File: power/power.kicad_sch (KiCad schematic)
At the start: 2 parts, among them J1 ET60T-D04-3-08-D04-X-R1-S, J2 796636-6

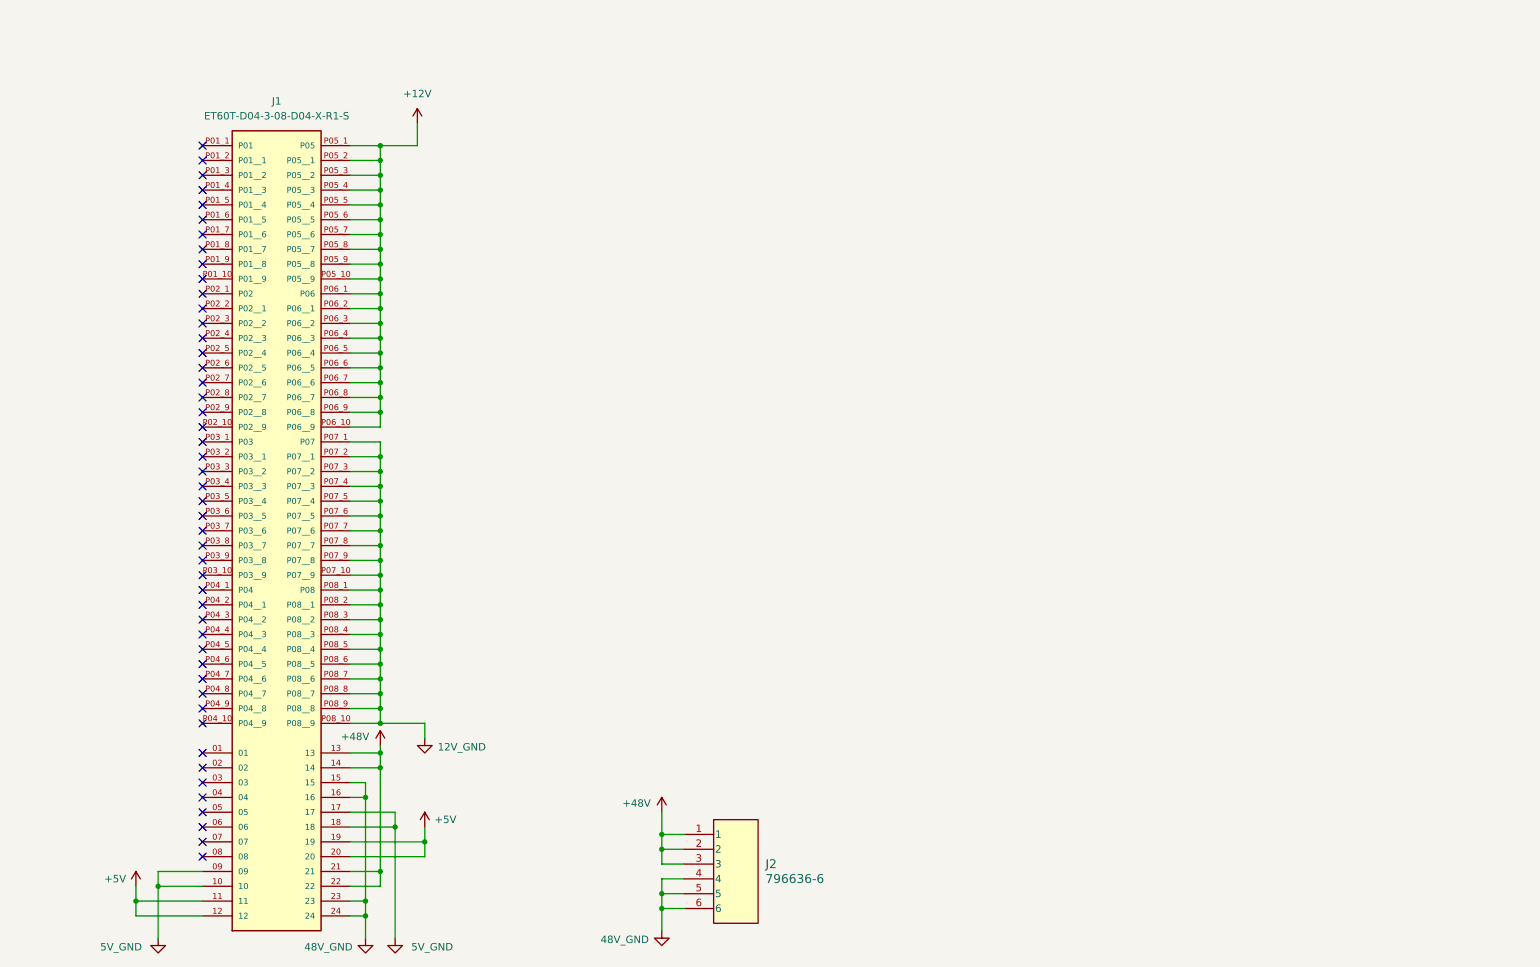
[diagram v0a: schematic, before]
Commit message: work
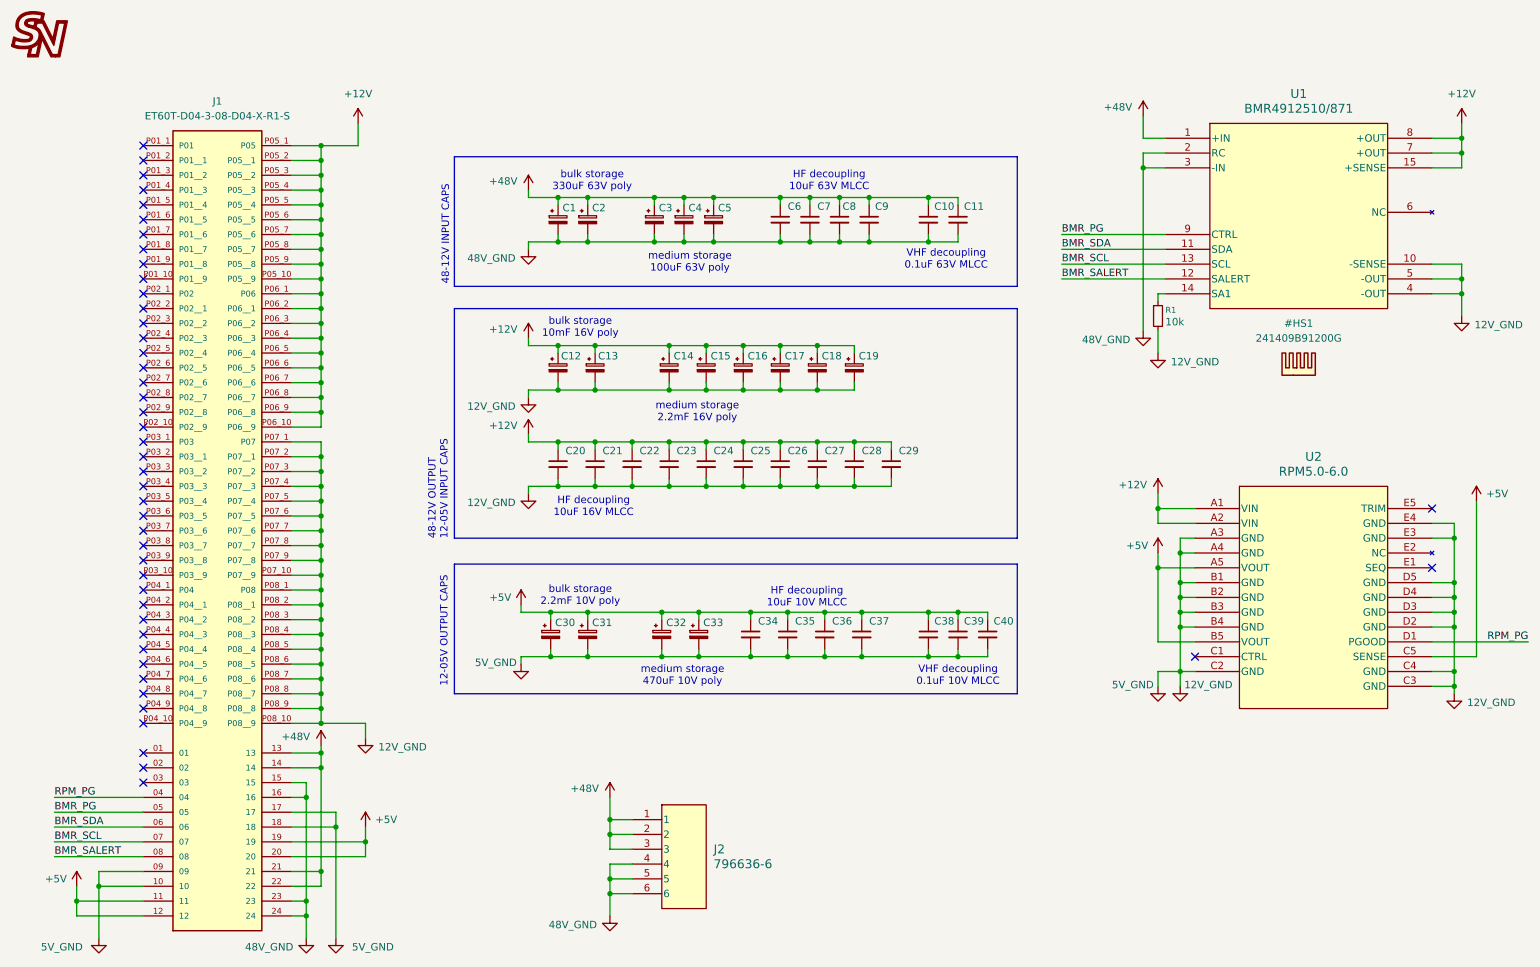
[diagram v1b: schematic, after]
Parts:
- added C1, C12, C13, C2: C_Polarized_Small, Capacitor_THT:CP_Radial_D18.0mm_P7.50mm, symbol Device:C_Polarized_Small
- added C10, C11, C20, C21, C22, C23, C24, C25, C26, C27, C28, C29, C34, C35, C36, C37, C38, C39, C40, C6, C7, C8, C9: C_Small, Capacitor_SMD:C_0603_1608Metric, symbol Device:C_Small
- added C14, C15, C16, C17, C18, C19, C30, C31, C32, C33: C_Polarized_Small, Capacitor_THT:CP_Radial_D10.0mm_P5.00mm, symbol Device:C_Polarized_Small
- added C3, C4, C5: C_Polarized_Small, Capacitor_THT:CP_Radial_D8.0mm_P5.00mm, symbol Device:C_Polarized_Small
- added G1: LOGO, custom:logo, symbol custom:LOGO
- added R1: 10k, Resistor_SMD:R_0603_1608Metric, symbol Device:R_Small
- added U1: BMR4912510/871, power_symbols:BMR491_FPM, symbol power_symbols:BMR4912510_871
- added U2: RPM5.0-6.0, power_symbols:RPM5.0-6.0, symbol power_symbols:RPM5.0-6.0
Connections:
- net 5V_GND is gone; now on net 12V_GND: J1.09, J1.10, J1.17, J1.18
- net +12V: now also C12.1, C13.1, C14.1, C15.1, C16.1, C17.1, C18.1, C19.1, C20.1, C21.1, C22.1, C23.1, C24.1, C25.1, C26.1, C27.1, C28.1, C29.1, U1.15 (+SENSE), U1.7 (+OUT), U1.8 (+OUT), U2.A1 (VIN), U2.A2 (VIN)
- net +48V: now also C1.1, C10.1, C11.1, C2.1, C3.1, C4.1, C5.1, C6.1, C7.1, C8.1, C9.1, U1.1 (+IN)
- net +5V: now also C30.1, C31.1, C32.1, C33.1, C34.1, C35.1, C36.1, C37.1, C38.1, C39.1, C40.1, U2.A5 (VOUT), U2.B5 (VOUT), U2.C5 (SENSE)
- net 12V_GND: now also C12.2, C13.2, C14.2, C15.2, C16.2, C17.2, C18.2, C19.2, C20.2, C21.2, C22.2, C23.2, C24.2, C25.2, C26.2, C27.2, C28.2, C29.2, C30.2, C31.2, C32.2, C33.2, C34.2, C35.2, C36.2, C37.2, C38.2, C39.2, C40.2, R1.2, U1.10 (-SENSE), U1.4 (-OUT), U1.5 (-OUT), U2.A3 (GND), U2.A4 (GND), U2.B1 (GND), U2.B2 (GND), U2.B3 (GND), U2.B4 (GND), U2.C2 (GND), U2.C3 (GND), U2.C4 (GND), U2.D2 (GND), U2.D3 (GND), U2.D4 (GND), U2.D5 (GND), U2.E3 (GND), U2.E4 (GND)
- net 48V_GND: now also C1.2, C10.2, C11.2, C2.2, C3.2, C4.2, C5.2, C6.2, C7.2, C8.2, C9.2, U1.2 (RC), U1.3 (-IN)
- net RPM_PG: now reaches J1.04
- net RPM_PG: now also U2.D1 (PGOOD)
- net BMR_PG: now reaches J1.05
- net BMR_PG: now also U1.9 (CTRL)
- net BMR_SDA: now reaches J1.06
- net BMR_SDA: now also U1.11 (SDA)
- net BMR_SCL: now reaches J1.07
- net BMR_SCL: now also U1.13 (SCL)
- net BMR_SALERT: now reaches J1.08
- net BMR_SALERT: now also U1.12 (SALERT)
- new net: R1.1, U1.14 (SA1)
- no-connect marks 48 -> 46
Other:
- note added: "12-05V OUTPUT CAPS"
- note added: "48-12V INPUT CAPS"
- note added: "48-12V OUTPUT 12-05V INPUT CAPS"
- note added: "HF decoupling 10uF 10V MLCC"
- note added: "HF decoupling 10uF 16V MLCC"
- note added: "HF decoupling 10uF 63V MLCC"
- note added: "VHF decoupling 0.1uF 10V MLCC"
- note added: "VHF decoupling 0.1uF 63V MLCC"
- note added: "bulk storage 10mF 16V poly"
- note added: "bulk storage 2.2mF 10V poly"
- note added: "bulk storage 330uF 63V poly"
- note added: "medium storage 100uF 63V poly"
- note added: "medium storage 2.2mF 16V poly"
- note added: "medium storage 470uF 10V poly"
- moved on the sheet: J1, J2
